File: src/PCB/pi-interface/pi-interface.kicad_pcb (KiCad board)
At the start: 2 copper layers, 21 x 19.1 mm, 4 parts, among them J1 PI

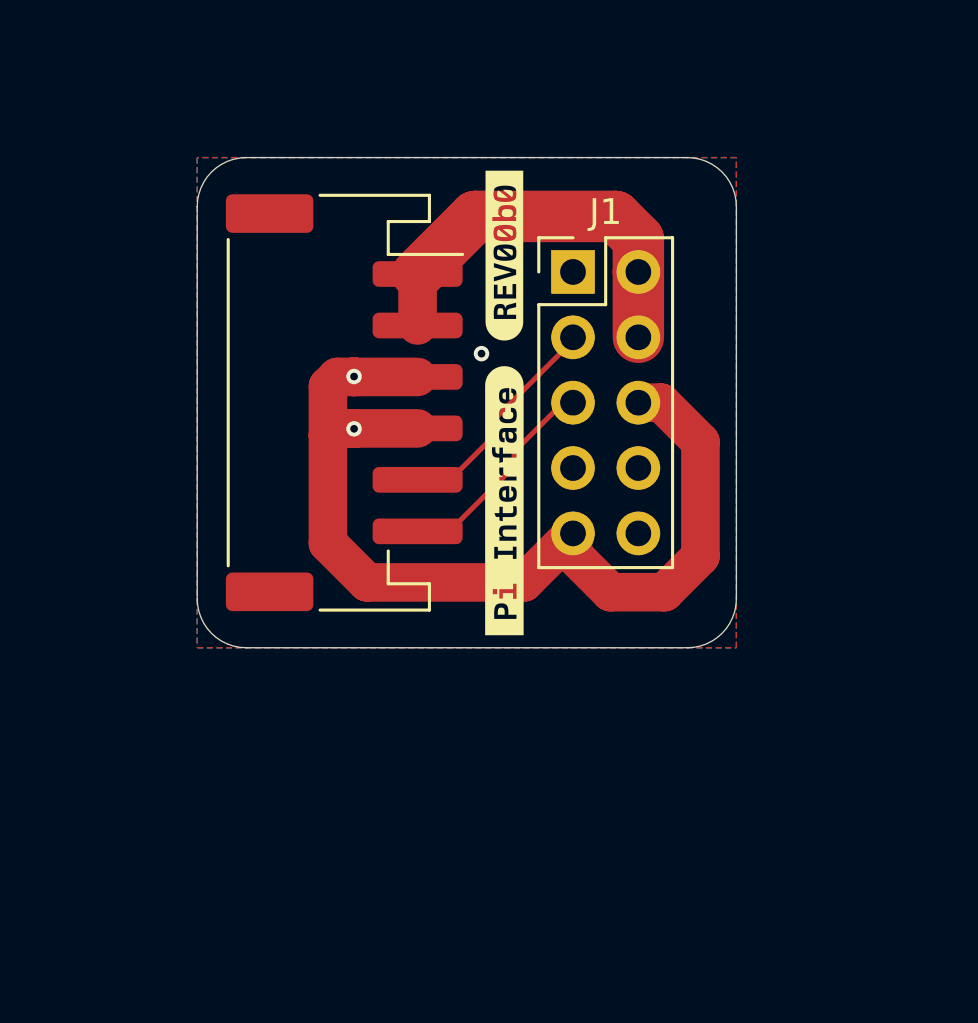
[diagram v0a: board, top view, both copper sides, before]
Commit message: updates readme image, offcenter cam cleanup
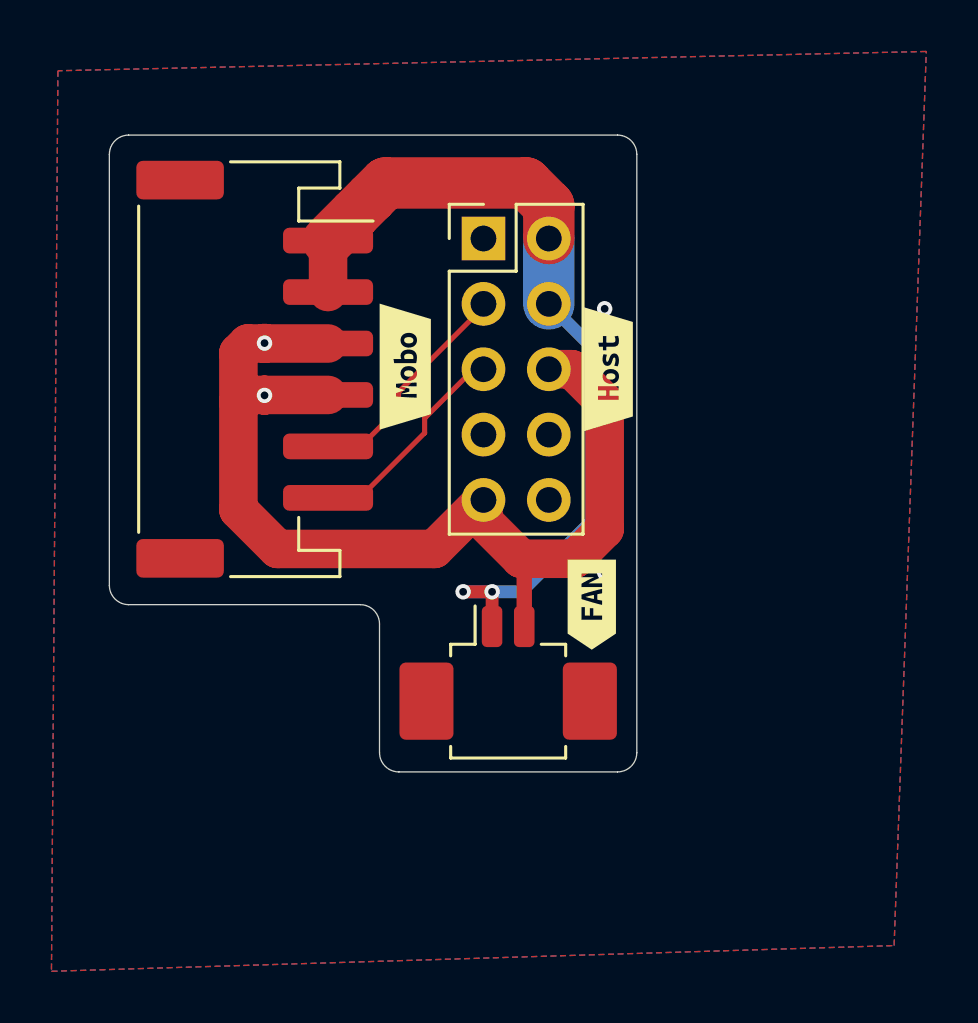
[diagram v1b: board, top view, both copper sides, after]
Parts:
- removed kibuzzard-6647A648: G***, kibuzzard-6647A648
- removed kibuzzard-6647A66F: G***, kibuzzard-6647A66F
- added J3: Conn_01x02_Pin, Connector_Molex:Molex_PicoBlade_53261-0271_1x02-1MP_P1.25mm_Horizontal, F.Cu at (30.5, 36.5)
- added kibuzzard-6ABE9D80: G***, kibuzzard-6ABE9D80, B.Cu at (23.6, 28.1)
- added kibuzzard-6ABE9DFF: G***, kibuzzard-6ABE9DFF, F.Cu at (33.8, 33.2)
- added kibuzzard-6ABE9E31: G***, kibuzzard-6ABE9E31, F.Cu at (26.5, 24.0)
- added kibuzzard-6ABE9E4D: G***, kibuzzard-6ABE9E4D, F.Cu at (34.4, 24.1)
- added kibuzzard-6ABE9EAF: G***, kibuzzard-6ABE9EAF, B.Cu at (21.2, 29.8)
- moved J1 3.71 mm to (29.5, 19.0)
- moved J2 3.71 mm to (20.6, 24.1)
- renumbered Je to J2
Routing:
- net +5V: track 15.7 -> 33.5 mm, vias 0 -> 2
- net GND: track 38.8 -> 41.2 mm, vias 3 -> 5
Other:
- board size 21 x 19.1 mm -> 20.5 x 24.8 mm
